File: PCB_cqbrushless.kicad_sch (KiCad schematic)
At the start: 40 parts, among them IC1 IR21834PBF, IC2 IR21834PBF, IC3 IR21834PBF, J1 B2B-XH-_MainSW, J2 B2B-XH_Direction, J3 B3B-XH_Accel, J4 B3B-XH_Ain, J5 B5B-XH_HallSens, Q1 2SK3711, Q2 2SK3711, Q3 2SK3711, Q4 2SK3711, Q5 2SK3711, Q6 2SK3711, U1 NCS3S1212SC

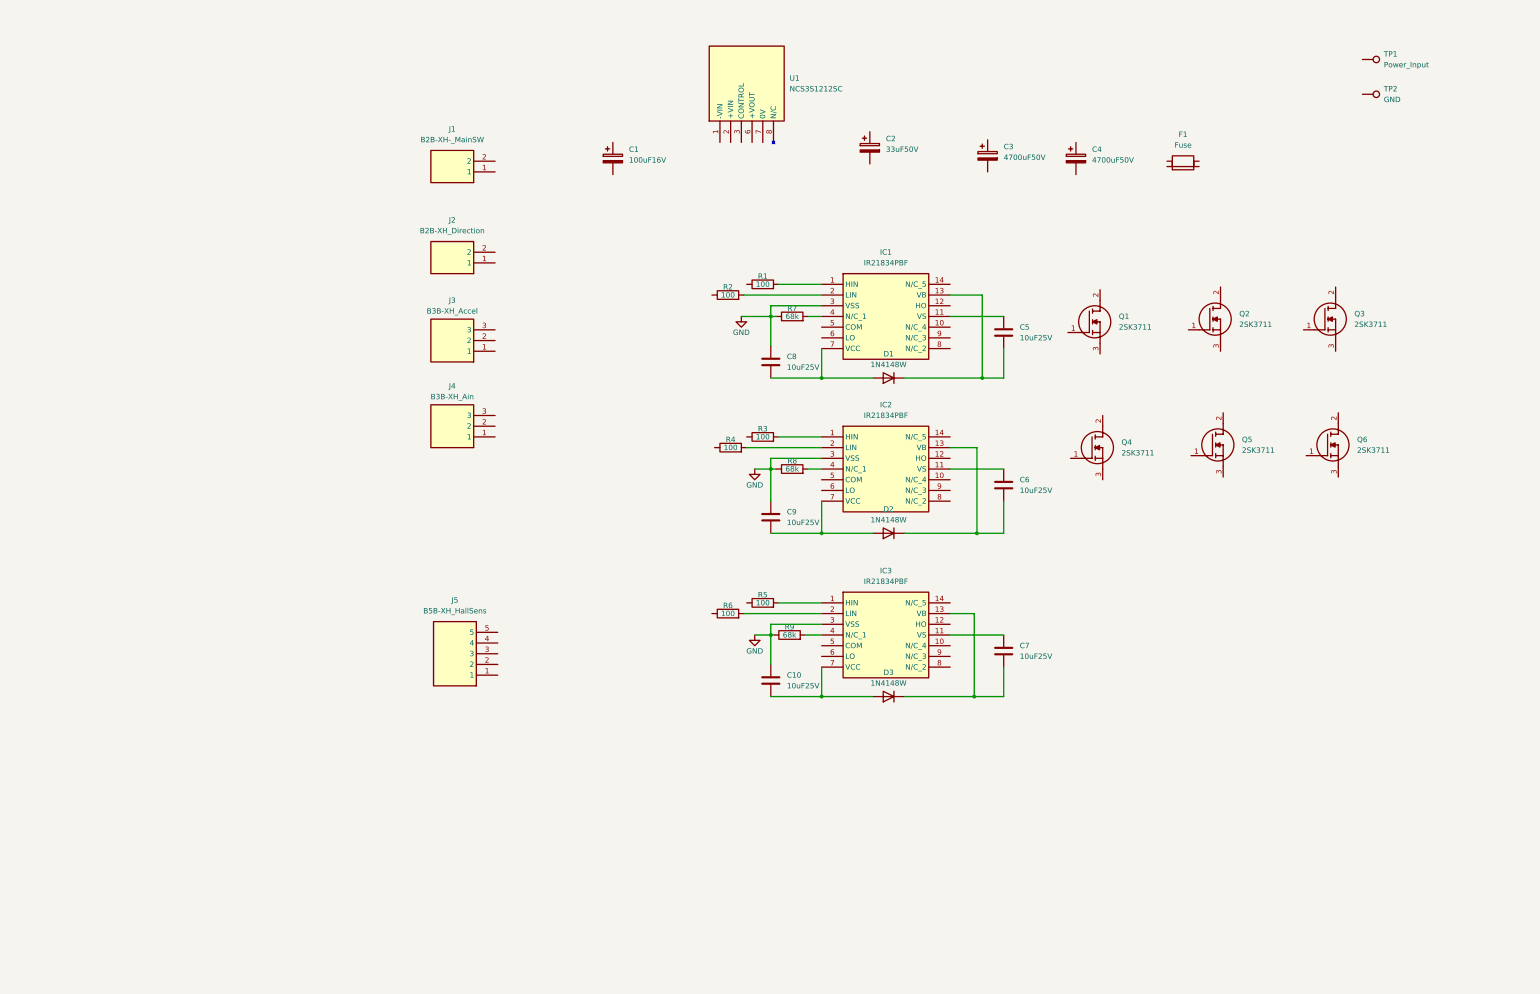
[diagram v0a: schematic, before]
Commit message: 0920
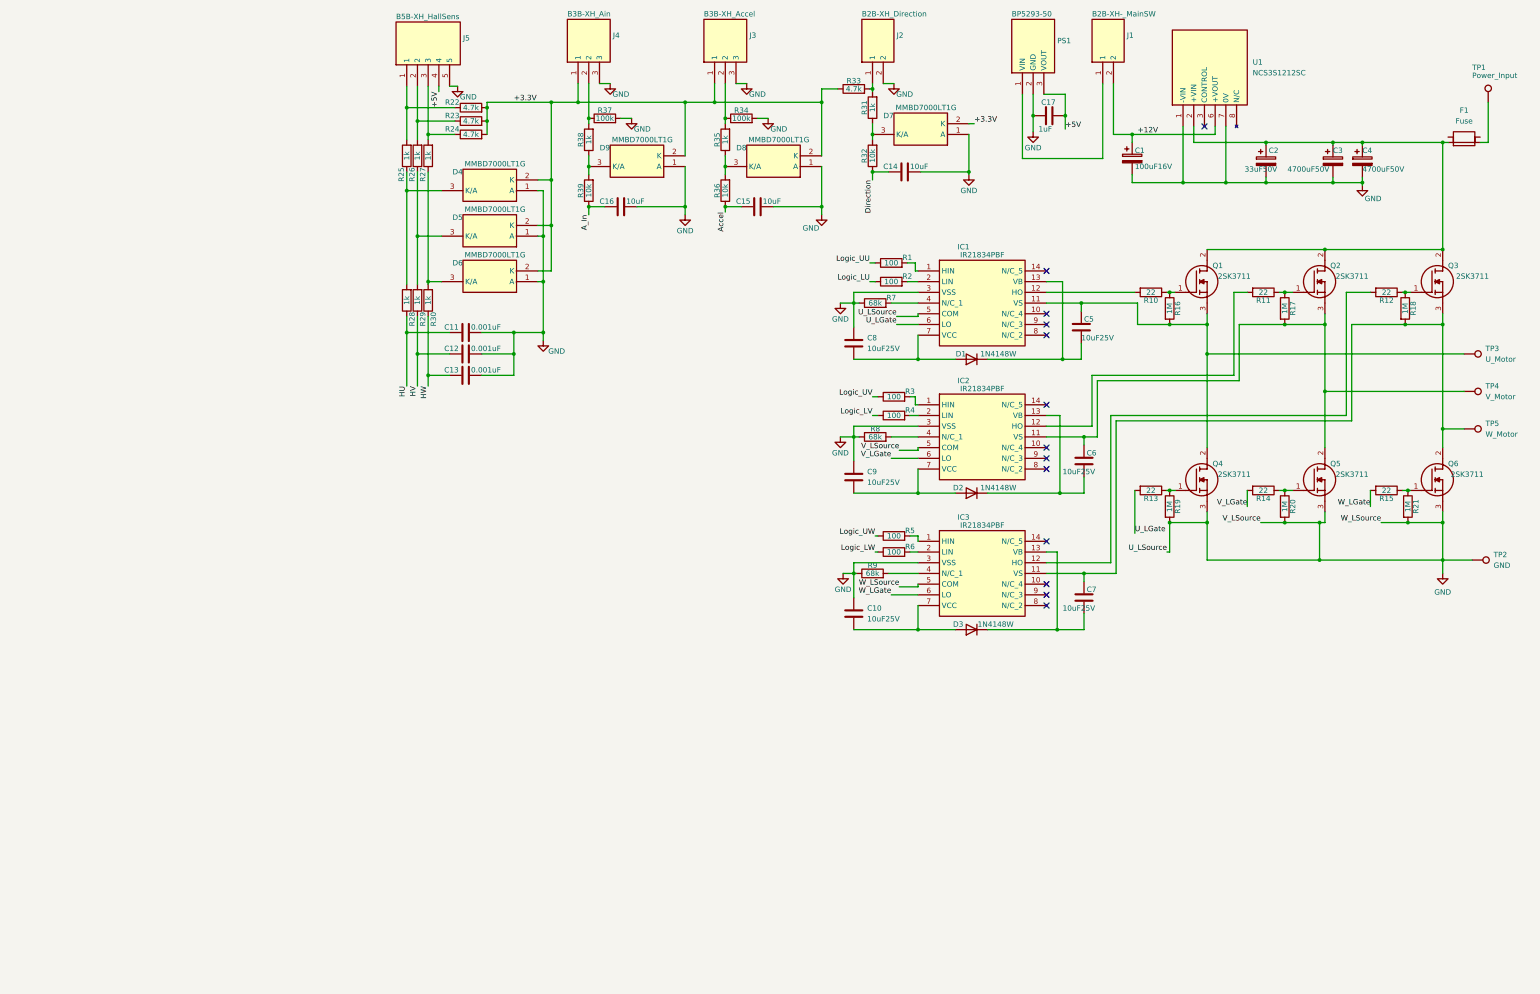
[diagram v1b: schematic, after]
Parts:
- added C11, C12, C13: 0.001uF, Capacitor_SMD:C_0603_1608Metric_Pad1.08x0.95mm_HandSolder, symbol Device:C
- added C14, C15, C16: 10uF, Capacitor_SMD:C_0603_1608Metric_Pad1.08x0.95mm_HandSolder, symbol Device:C
- added C17: 1uF, Capacitor_SMD:C_0603_1608Metric_Pad1.08x0.95mm_HandSolder, symbol Device:C
- added D4, D5, D6, D7, D8, D9: MMBD7000LT1G, SOT96P237X111-3N, symbol SamacSys_Parts:MMBD7000LT1G
- added PS1: BP5293-50, TO254P570X1700X1780-3P, symbol SamacSys_Parts:BP5293-50
- added R10, R11, R12, R13, R14, R15: 22, Resistor_SMD:R_0603_1608Metric_Pad0.98x0.95mm_HandSolder, symbol Device:R
- added R16, R17, R18, R19, R20, R21: 1M, Resistor_SMD:R_0603_1608Metric_Pad0.98x0.95mm_HandSolder, symbol Device:R
- added R22, R23, R24, R33: 4.7k, Resistor_SMD:R_0603_1608Metric_Pad0.98x0.95mm_HandSolder, symbol Device:R
- added R25, R26, R27, R28, R29, R30, R31, R35, R38: 1k, Resistor_SMD:R_0603_1608Metric_Pad0.98x0.95mm_HandSolder, symbol Device:R
- added R32, R36, R39: 10k, Resistor_SMD:R_0603_1608Metric_Pad0.98x0.95mm_HandSolder, symbol Device:R
- added R34, R37: 100k, Resistor_SMD:R_0603_1608Metric_Pad0.98x0.95mm_HandSolder, symbol Device:R
- added TP3: U_Motor, MountingHole:MountingHole_3.7mm_Pad, symbol Connector:TestPoint
- added TP4: V_Motor, MountingHole:MountingHole_3.7mm_Pad, symbol Connector:TestPoint
- added TP5: W_Motor, MountingHole:MountingHole_3.7mm_Pad, symbol Connector:TestPoint
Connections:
- net GND: now also C1.2, C2.2, C3.2, C4.2, IC1.5 (COM), IC2.5 (COM), IC3.5 (COM), J2.2, J3.3, J4.3, J5.5, Q4.3 (S), Q5.3 (S), Q6.3 (S), TP2.1, U1.1 (-VIN), U1.7 (0V), C11.1, C12.1, C13.1, C14.1, C15.1, C16.1, C17.2, D4.1 (A), D5.1 (A), D6.1 (A), D7.1 (A), D8.1 (A), D9.1 (A), PS1.2 (GND), R19.2, R20.2, R21.2, R34.2, R37.2
- net at Q1.1 (G): now also R10.1, R16.1
- net at Q1.2 (D): now also C2.1, C3.1, C4.1, F1.1, Q2.2 (D), Q3.2 (D), U1.2 (+VIN)
- net at Q1.3 (S): now also C5.1, IC1.11 (VS), Q4.2 (D), R16.2, TP3.1
- net Logic_LV: now reaches R4.1
- net +3.3V: now reaches J3.1
- net +3.3V: now also J4.1, D4.2 (K), D5.2 (K), D6.2 (K), D7.2 (K), D8.2 (K), D9.2 (K), R22.2, R23.2, R24.2, R33.1
- net at J3.2: now also R34.1, R35.2
- net at J2.1: now also R31.2, R33.2
- net at C6.1, IC2.11 (VS): now also Q2.3 (S), Q5.2 (D), R17.2, TP4.1
- net Logic_UU: now reaches R1.1
- net at Q4.1 (G): now also R13.1, R19.1
- net at Q6.1 (G): now also R15.1, R21.1
- net at Q6.2 (D): now also C7.1, IC3.11 (VS), Q3.3 (S), R18.2, TP5.1
- net Logic_LW: now reaches R6.1
- net Logic_LU: now reaches R2.1
- net at Q5.1 (G): now also R14.1, R20.1
- net Logic_UW: now reaches R5.1
- net at J4.2: now also R37.1, R38.2
- net +12V: now reaches C1.1
- net +12V: now also J1.2, U1.6 (+VOUT)
- net at IC1.12 (HO): now also R10.2
- net U_LGate: now reaches IC1.6 (LO)
- net U_LGate: now also R13.2
- net at J5.1: now also R22.1, R25.2
- net at J5.2: now also R23.1, R26.2
- net at J5.3: now also R24.1, R27.2
- net +5V: now reaches J5.4
- net +5V: now also C17.1, PS1.3 (VOUT)
- net Logic_UV: now reaches R3.1
- net at Q2.1 (G): now also R11.1, R17.1
- net at F1.3: now also TP1.1
- net at IC2.12 (HO): now also R11.2
- net V_LGate: now reaches IC2.6 (LO)
- net V_LGate: now also R14.2
- net at Q3.1 (G): now also R12.1, R18.1
- net at IC3.12 (HO): now also R12.2
- net W_LGate: now reaches IC3.6 (LO)
- net W_LGate: now also R15.2
- net at J1.1: now also PS1.1 (VIN)
- new net: D4.3 (K/A), R25.1, R28.2
- new net: D7.3 (K/A), R31.1, R32.2
- new net: D5.3 (K/A), R26.1, R29.2
- new net: D6.3 (K/A), R27.1, R30.2
- new net: D8.3 (K/A), R35.1, R36.2
- new net: D9.3 (K/A), R38.1, R39.2
- new net A_In: C16.2, R39.1
- new net Accel: C15.2, R36.1
- new net Direction: C14.2, R32.1
- new net HU: C11.2, R28.1
- new net HV: C12.2, R29.1
- new net HW: C13.2, R30.1
- no-connect marks 0 -> 13
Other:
- moved on the sheet: C1, C10, C2, C3, C4, C5, C6, C7, C8, C9, D1, D2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

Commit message: 0925
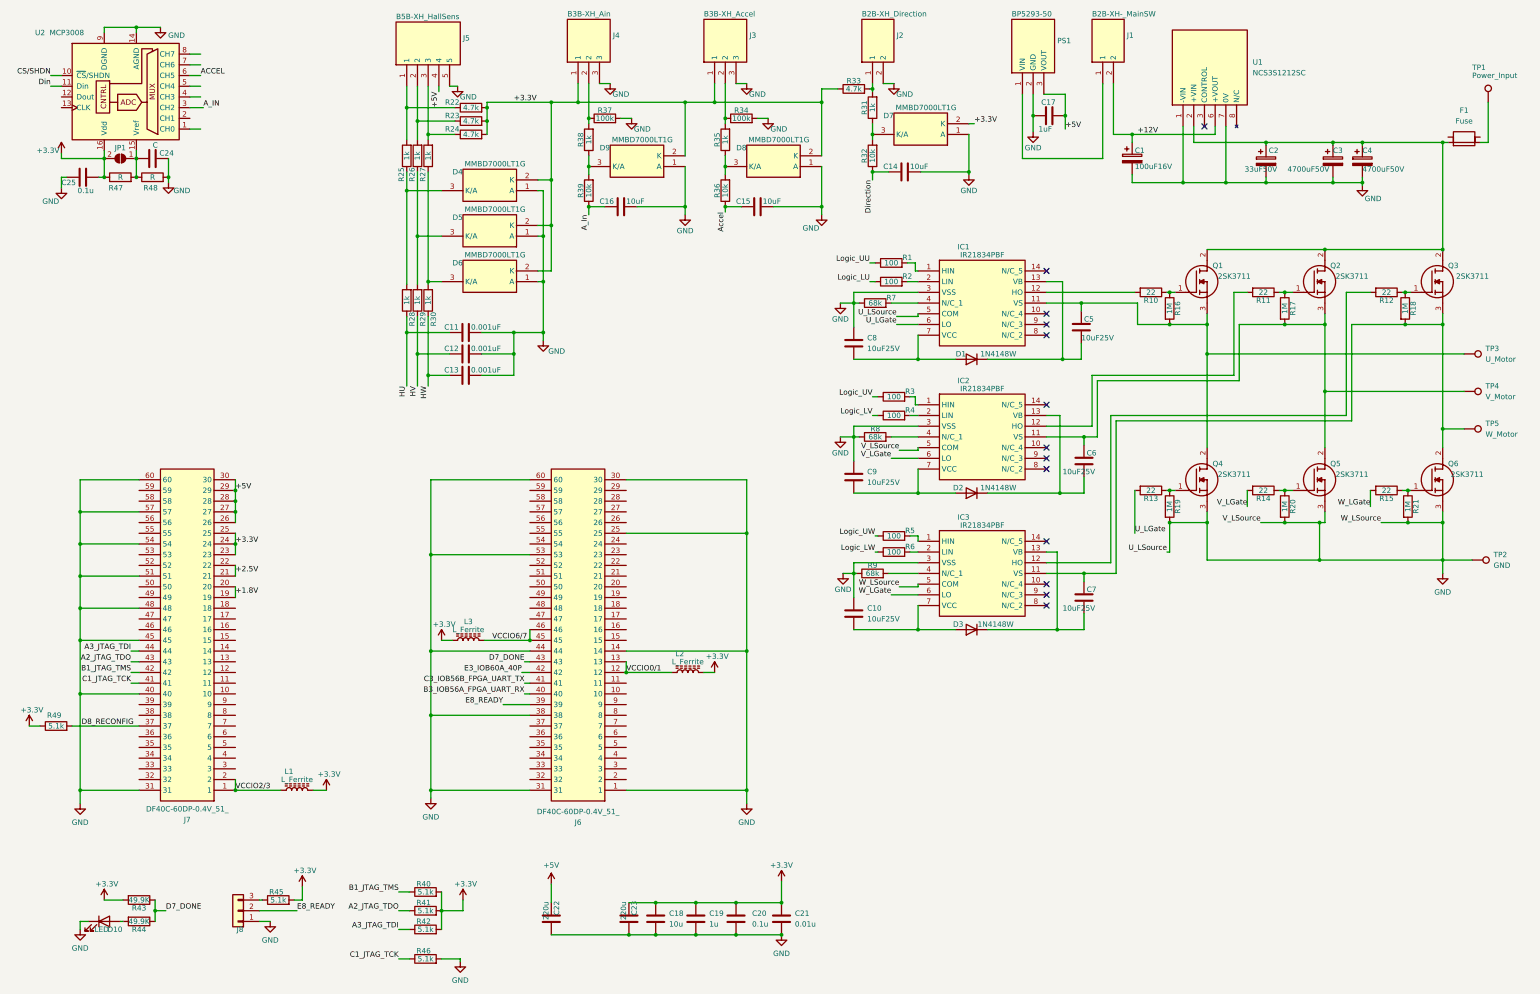
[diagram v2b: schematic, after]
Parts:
- added C18: 10u, Capacitor_SMD:C_1206_3216Metric_Pad1.33x1.80mm_HandSolder, symbol Device:C
- added C19: 1u, Capacitor_SMD:C_0603_1608Metric_Pad1.08x0.95mm_HandSolder, symbol Device:C
- added C20, C25: 0.1u, Capacitor_SMD:C_0603_1608Metric_Pad1.08x0.95mm_HandSolder, symbol Device:C
- added C21: 0.01u, Capacitor_SMD:C_0603_1608Metric_Pad1.08x0.95mm_HandSolder, symbol Device:C
- added C22, C23: 220u, Capacitor_SMD:C_1206_3216Metric_Pad1.33x1.80mm_HandSolder, symbol Device:C
- added C24: C, Capacitor_SMD:C_0603_1608Metric_Pad1.08x0.95mm_HandSolder, symbol Device:C
- added D10: LED, LED_SMD:LED_0603_1608Metric_Pad1.05x0.95mm_HandSolder, symbol Device:LED
- added J6, J7: DF40C-60DP-0.4V_51_, DF40C-60DP-0.4V(51), symbol SamacSys_Parts:DF40C-60DP-0.4V_51_
- added J8: Conn_01x03, Connector_PinHeader_2.54mm:PinHeader_1x03_P2.54mm_Vertical, symbol Connector_Generic:Conn_01x03
- added JP1: SolderJumper_2_Open, Jumper:SolderJumper-2_P1.3mm_Open_TrianglePad1.0x1.5mm, symbol Jumper:SolderJumper_2_Open
- added L1, L2, L3: L_Ferrite, Inductor_SMD:L_0603_1608Metric_Pad1.05x0.95mm_HandSolder, symbol Device:L_Ferrite
- added R40, R41, R42, R45, R46, R49: 5.1k, Resistor_SMD:R_0603_1608Metric_Pad0.98x0.95mm_HandSolder, symbol Device:R
- added R43, R44: 49.9K, Resistor_SMD:R_0603_1608Metric_Pad0.98x0.95mm_HandSolder, symbol Device:R
- added R47, R48: R, Resistor_SMD:R_0603_1608Metric_Pad0.98x0.95mm_HandSolder, symbol Device:R
- added U2: MCP3008, Package_DIP:DIP-16_W7.62mm, symbol Analog_ADC:MCP3008
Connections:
- net +3.3V: now also C18.1, C19.1, C20.1, C21.1, C23.1, C25.1, J7.23, J7.24, J7.25, JP1.2 (B), L1.2, L2.2, L3.1, R40.2, R41.2, R42.2, R43.2, R45.2, R47.1, R49.1, U2.16 (Vdd)
- net +5V: now also C22.1, J7.26, J7.27, J7.28, J7.29, J7.30
- net GND: now also C18.2, C19.2, C20.2, C21.2, C22.2, C23.2, C24.2, C25.2, D10.1 (K), J6.1, J6.14, J6.25, J6.30, J6.31, J6.38, J6.44, J6.53, J6.60, J7.31, J7.40, J7.45, J7.48, J7.51, J7.54, J7.57, J7.60, J8.1 (Pin_1), R46.2, R48.2, U2.14 (AGND), U2.9 (DGND)
- new net: C24.1, JP1.1 (A), R47.2, R48.1, U2.15 (Vref)
- new net: D10.2 (A), R44.2
- new net: J8.3 (Pin_3), R45.1
- new net +1.8V: J7.19, J7.20
- new net +2.5V: J7.21, J7.22
- new net A2_JTAG_TDO: J7.43, R41.1
- new net A3_JTAG_TDI: J7.44, R42.1
- new net ACCEL: U2.6 (CH5)
- new net A_IN: U2.3 (CH2)
- new net B1_JTAG_TMS: J7.42, R40.1
- new net B3_IOB56A_FPGA_UART_RX: J6.40
- new net C1_JTAG_TCK: J7.41, R46.1
- new net C3_IOB56B_FPGA_UART_TX: J6.41
- new net CS/SHDN: U2.10 (~{CS}/SHDN)
- new net D7_DONE: J6.43, R43.1, R44.1
- new net D8_RECONFIG: J7.37, R49.2
- new net Din: U2.11 (Din)
- new net E3_IOB60A_40P: J6.42
- new net E8_READY: J6.39, J8.2 (Pin_2)
- new net VCCIO0/1: J6.12, J6.13, L2.1
- new net VCCIO2/3: J7.1, J7.2, L1.1
- new net VCCIO6/7: J6.45, J6.46, L3.2
